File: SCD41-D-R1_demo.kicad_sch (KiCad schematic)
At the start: 11 parts, among them J1 USB_A, U1 SCD41-D-R2, U2 AP2112K-3.3, U3 USBLC6-2SC6

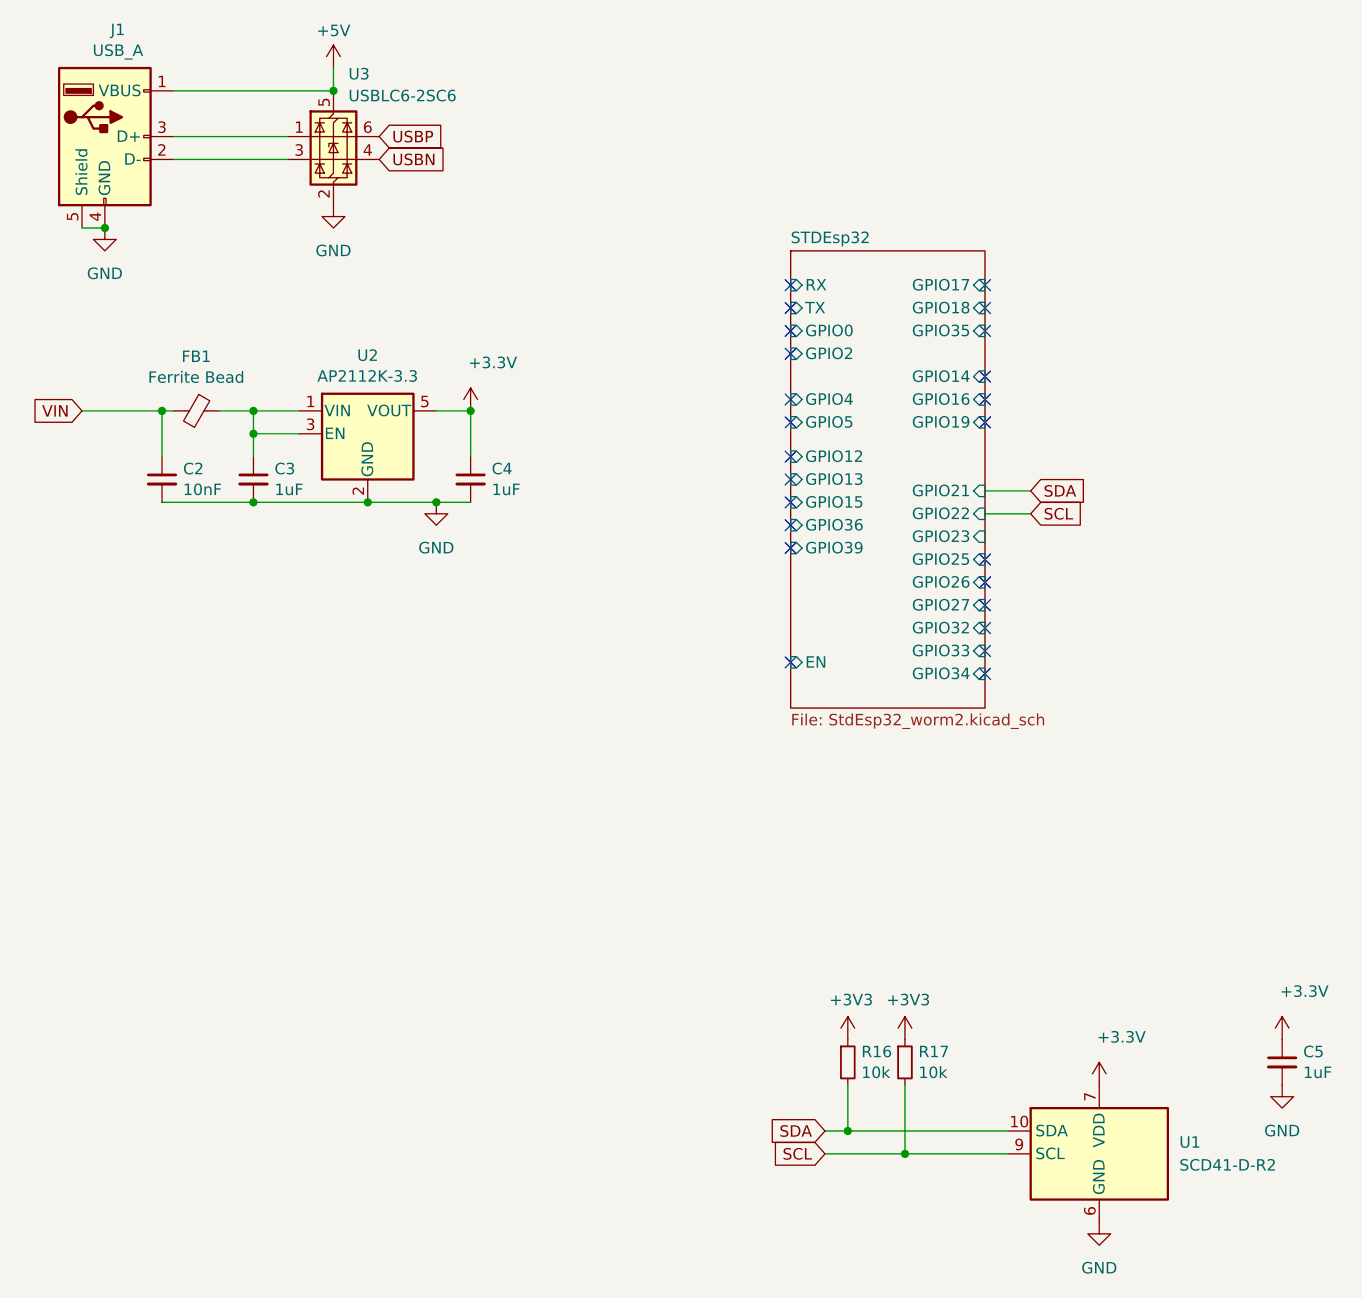
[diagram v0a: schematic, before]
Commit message: programmer
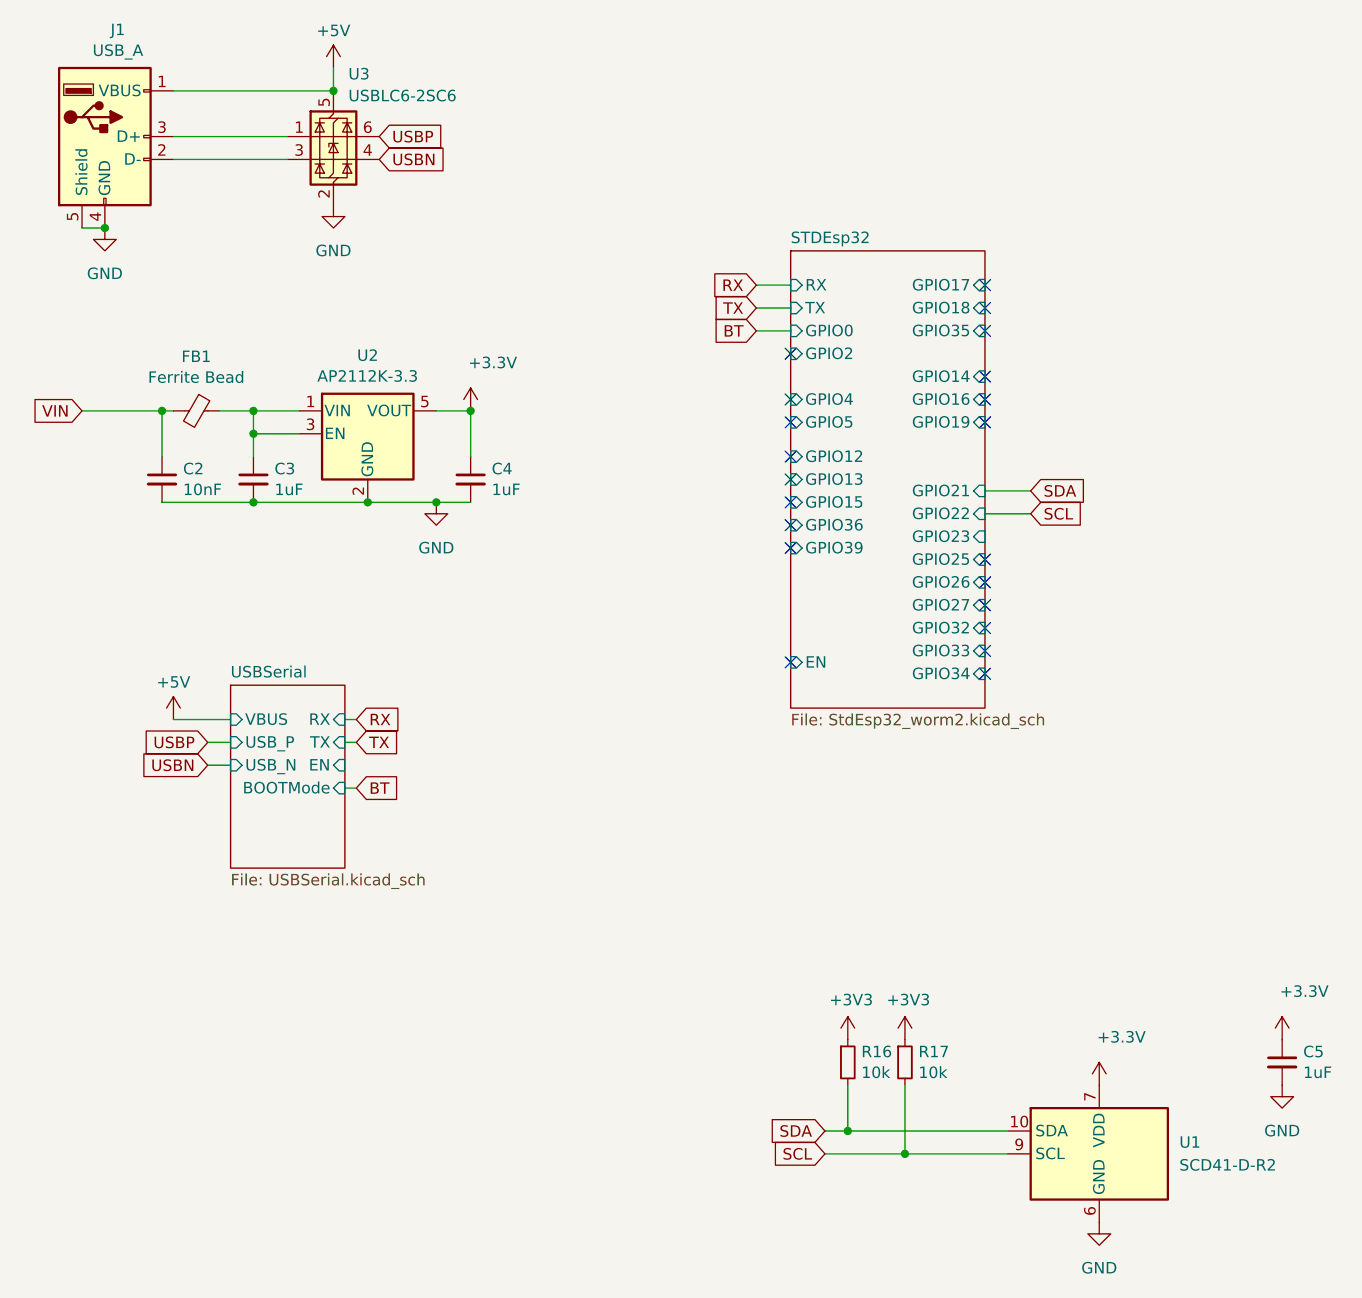
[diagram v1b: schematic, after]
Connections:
- no-connect marks 24 -> 21
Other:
- added sheet USBSerial (USBSerial.kicad_sch)
